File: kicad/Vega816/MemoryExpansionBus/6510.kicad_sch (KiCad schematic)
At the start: 26 parts, among them J0A1 Conn_02x40_Odd_Even, J0B1 CPU, J43 VPA/VDA, J44 ~{IO_AREA_OUT}

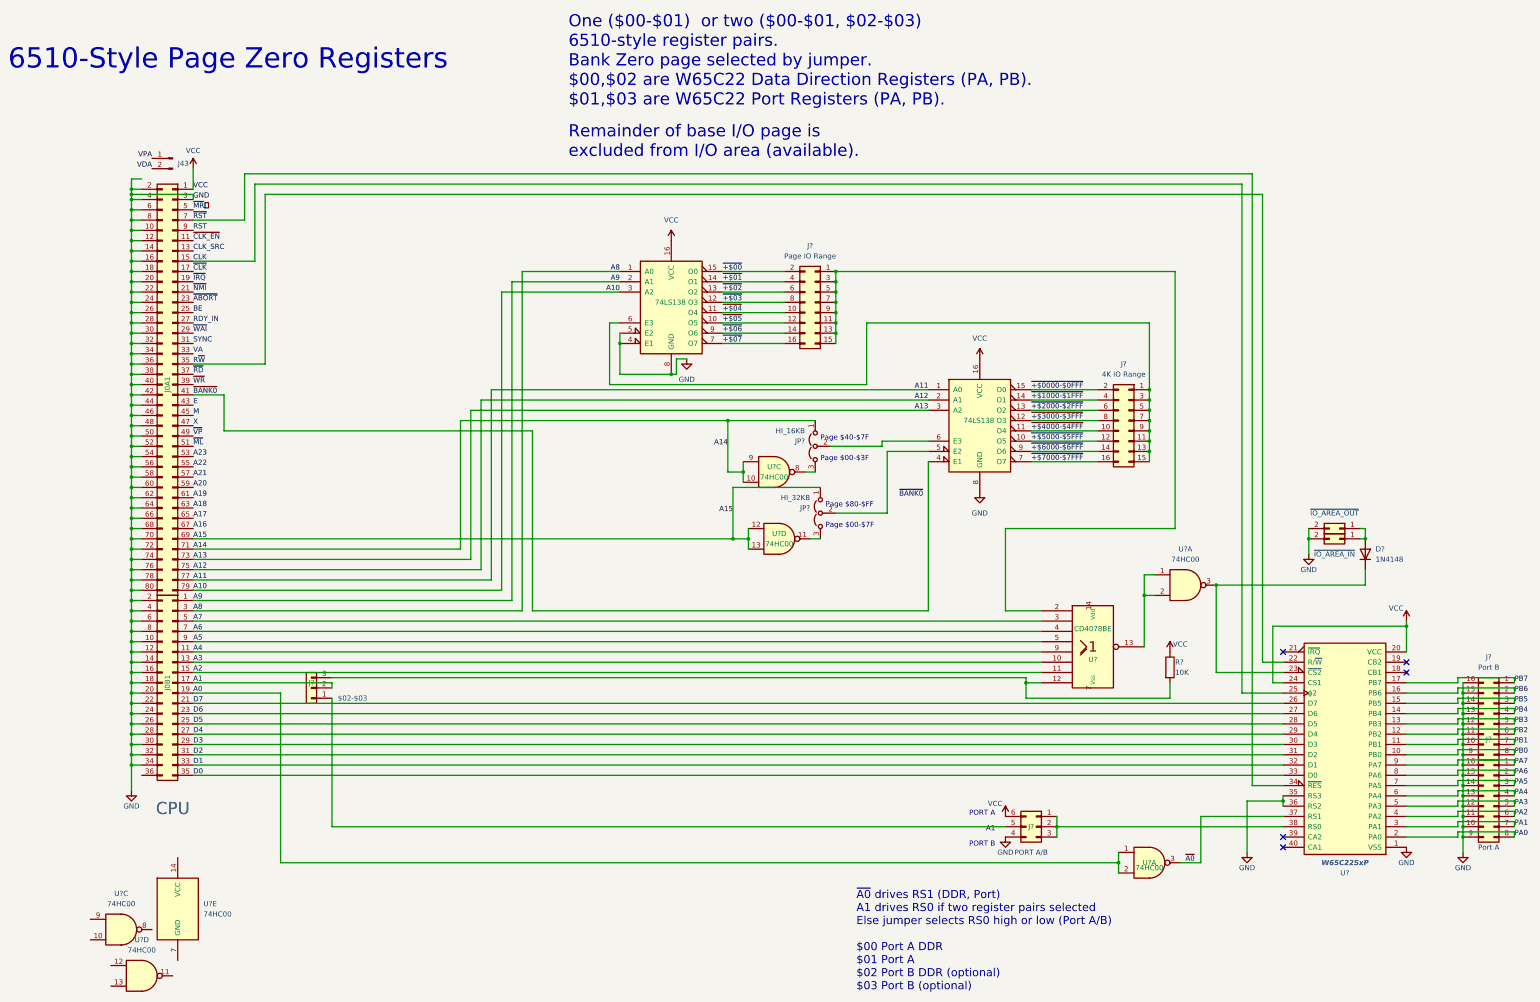
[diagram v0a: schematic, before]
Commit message: Big push, Sysctl, DMA Reg
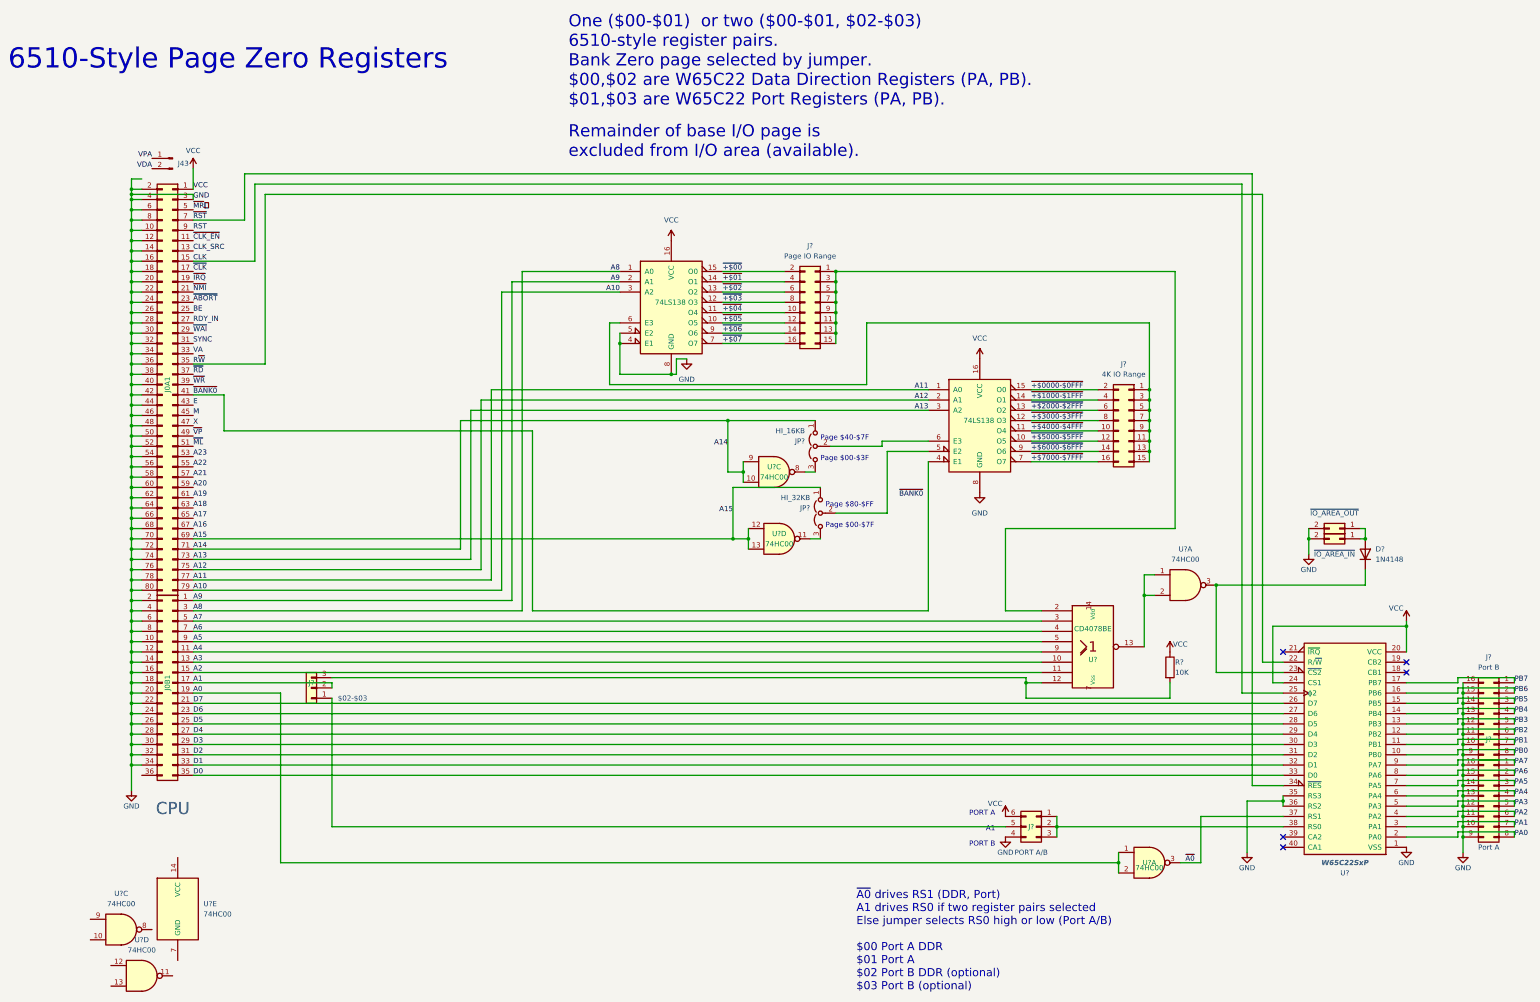
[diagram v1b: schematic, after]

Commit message: dfsg
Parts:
- removed D?: 1N4148, Diode_THT:D_DO-35_SOD27_P7.62mm_Horizontal, symbol Diode:1N4148
- removed J0A1: Conn_02x40_Odd_Even, Connector_PinHeader_2.54mm:PinHeader_2x40_P2.54mm_Vertical, symbol Connector_Generic:Conn_02x40_Odd_Even
- removed J0B1: CPU, Connector_PinHeader_2.54mm:PinHeader_2x18_P2.54mm_Vertical, symbol Connector_Generic:Conn_02x18_Odd_Even
- removed J43: VPA/VDA, symbol Connector:Conn_01x02_Male
- removed J44: ~{IO_AREA_OUT}, symbol Connector_Generic:Conn_02x01
- removed J?: ~{IO_AREA_IN}, symbol Connector_Generic:Conn_02x01
- removed J?: Page IO Range, symbol Connector_Generic:Conn_02x08_Odd_Even
- removed J?: Port B, symbol Connector_Generic:Conn_02x08_Counter_Clockwise
- removed J?: 4K IO Range, symbol Connector_Generic:Conn_02x08_Odd_Even
- removed J?: PORT A/B, symbol Connector_Generic:Conn_02x03_Counter_Clockwise
- removed J?: Port A, symbol Connector_Generic:Conn_02x08_Counter_Clockwise
- removed J?: $02-$03, symbol Connector_Generic:Conn_01x03
- removed JP?: HI_16KB, symbol Jumper:Jumper_3_Open
- removed JP?: HI_32KB, symbol Jumper:Jumper_3_Open
- removed R?: 10K, symbol Device:R
- removed U? (x2): 74LS138, symbol 74xx:74LS138
- removed U? (x7): 74HC00, symbol 74xx:74HC00
- removed U?: W65C22SxP, Package_DIP:DIP-40_W15.24mm_Socket, symbol Vega816:W65C22SxP
- removed U?: CD4078BE, symbol Vega816:CD4078BE
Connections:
- no-connect marks 5 -> 0
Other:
- note removed: "6510-Style Page Zero Registers"
- note removed: "A1"
- note removed: "One ($00-$01) or two ($00-$01, $02-$03) 6510-style register pairs. Bank Zero page selected by jumper. $00,$02 are W65C22 Data Direction Registers (PA, PB). $01,$03 are W65C22 Port Registers (PA, PB)."
- note removed: "PORT A"
- note removed: "PORT B"
- note removed: "Page $00-$3F"
- note removed: "Page $00-$7F"
- note removed: "Page $40-$7F"
- note removed: "Page $80-$FF"
- note removed: "Remainder of base I/O page is excluded from I/O area (available)."
- note removed: "~{A0} drives RS1 (DDR, Port) A1 drives RS0 if two register pairs selected Else jumper selects RS0 high or low (Port A/B) $00 Port A DDR $01 Port A $02 Port B DDR (optional) $03 Port B (optional)"
